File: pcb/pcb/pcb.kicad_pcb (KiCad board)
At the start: 2 copper layers, 130 x 80 mm, 30 parts, among them J1 SD Card, J2 Mic, J3 Relay Solenoid, J4 Status LED, P1 Power, SW1 Button Up, SW2 Button Down, SW3 Button Record, SW4 Button Delete, SW5 Button Play

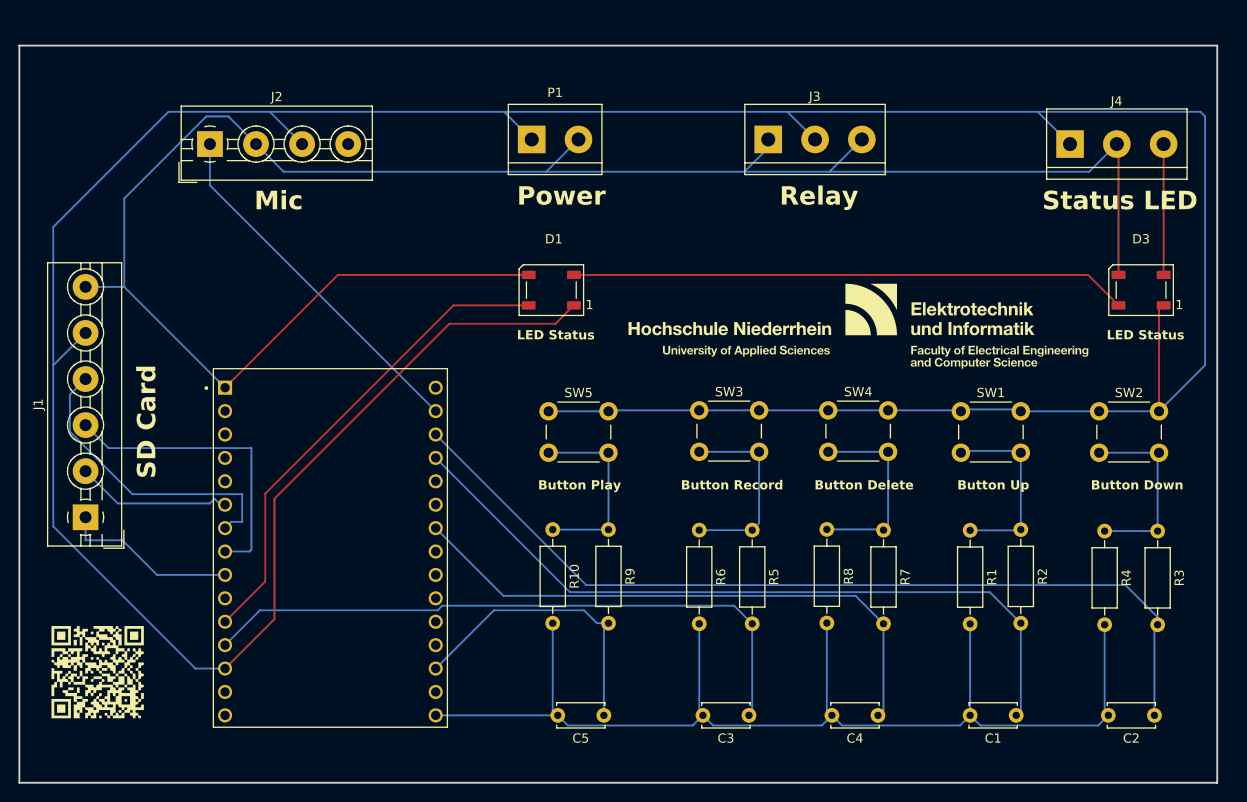
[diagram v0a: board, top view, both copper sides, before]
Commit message: Finish 100x80
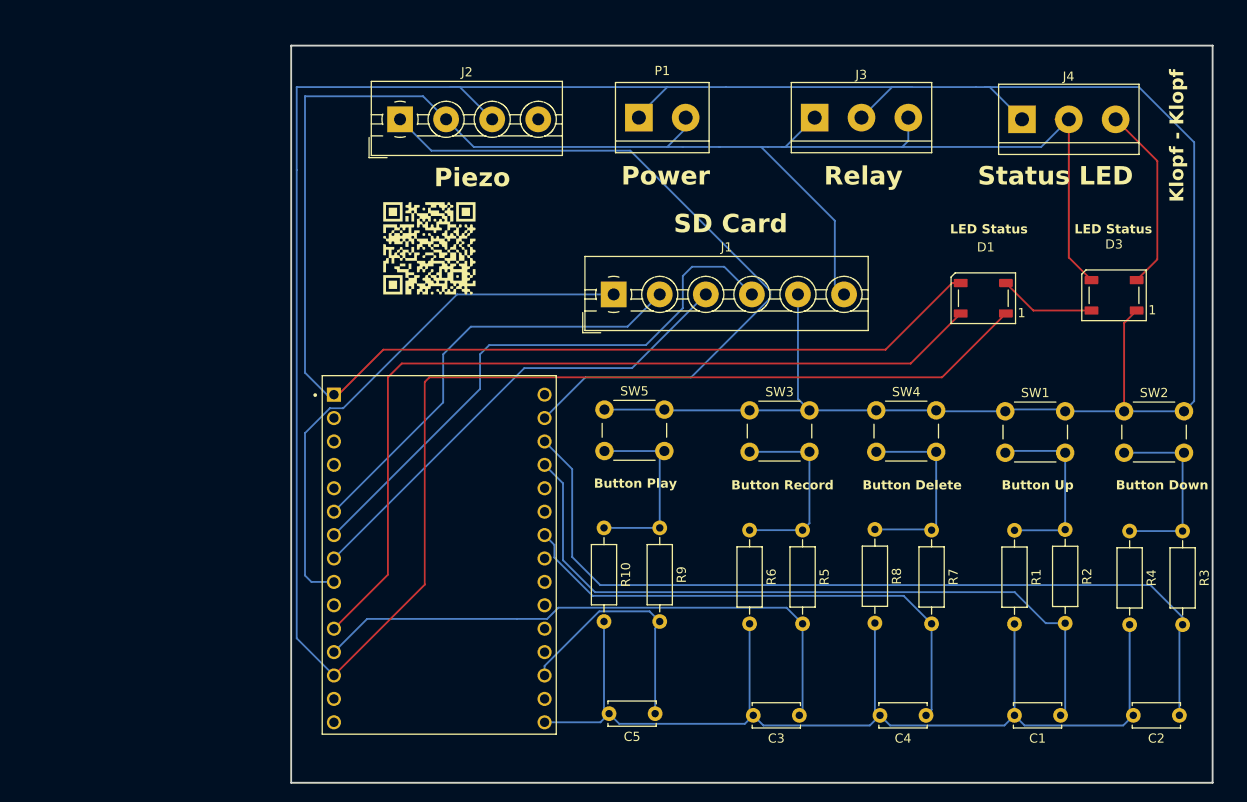
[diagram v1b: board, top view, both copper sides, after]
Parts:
- G***: moved to B.Cu
- moved J1 62.2 mm to (134.5, 77.5), turned to 0 degrees
- moved G*** 58.4 mm to (114.5, 72.5)
- moved D1 46.9 mm to (174.6, 77.9)
- moved J2 20.8 mm to (111.3, 58.5)
- moved G*** 15.9 mm to (171.5, 69.0), turned to 180 degrees
- moved P1 11.9 mm to (137.2, 58.3)
- moved REF** 11.8 mm to (115.6, 105.8)
- moved SW5 6.07 mm to (133.5, 90.0)
- moved J4 5.86 mm to (178.8, 58.5)
- moved J3 5.57 mm to (156.3, 58.3)
- moved C5 5.57 mm to (139.0, 123.0)
- moved R9 5.57 mm to (139.5, 102.8)
- moved R10 5.57 mm to (133.4, 102.8)
- moved C3 5.47 mm to (154.7, 123.2)
- moved R5 5.47 mm to (155.0, 103.1)
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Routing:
- net Net-(D1-DOUT): track 60.5 -> 10.5 mm
- net Net-(D1-DIN): track 52.8 -> 94.7 mm
- net Net-(J1-CS): track 19.2 -> 58.6 mm
- net Net-(J2-A0): track 39.8 -> 78.6 mm
- net Net-(J1-SCK): track 17.1 -> 48.2 mm
- net Net-(J1-MISO): track 33.1 -> 62.9 mm
- net GND: track 339.5 -> 363.2 mm
- net 5V: track 385.3 -> 407.9 mm
- net Net-(J1-MOSI): track 33.0 -> 52.2 mm
- net Net-(U1-GPIO9): track 70.2 -> 64.0 mm
- net Net-(U1-GPIO10): track 63.1 -> 57.0 mm
- net Net-(D3-DOUT): track 14.2 -> 20.3 mm
- net Net-(U1-GPIO19/USBD_+): track 32.9 -> 27.4 mm
- net Net-(U1-GPIO1): track 97.4 -> 93.5 mm
- net Net-(U1-GPIO2): track 81.1 -> 78.7 mm
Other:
- board size 130 x 80 mm -> 100 x 80 mm
- board text added: "Group 9"
- board text added: "Klopf - Klopf"
- board text added: "Piezo"
- board text removed: "Mic"
